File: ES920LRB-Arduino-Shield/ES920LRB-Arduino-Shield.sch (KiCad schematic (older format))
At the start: 18 parts, among them J1 Conn_01x10_Female, J2 Conn_01x12_Female, M1 ES920LR2B, P1 Power, P2 Analog, P3 Digital, P4 Digital, P5 CONN_01X01, P6 CONN_01X01, P7 CONN_01X01, P8 CONN_01X01

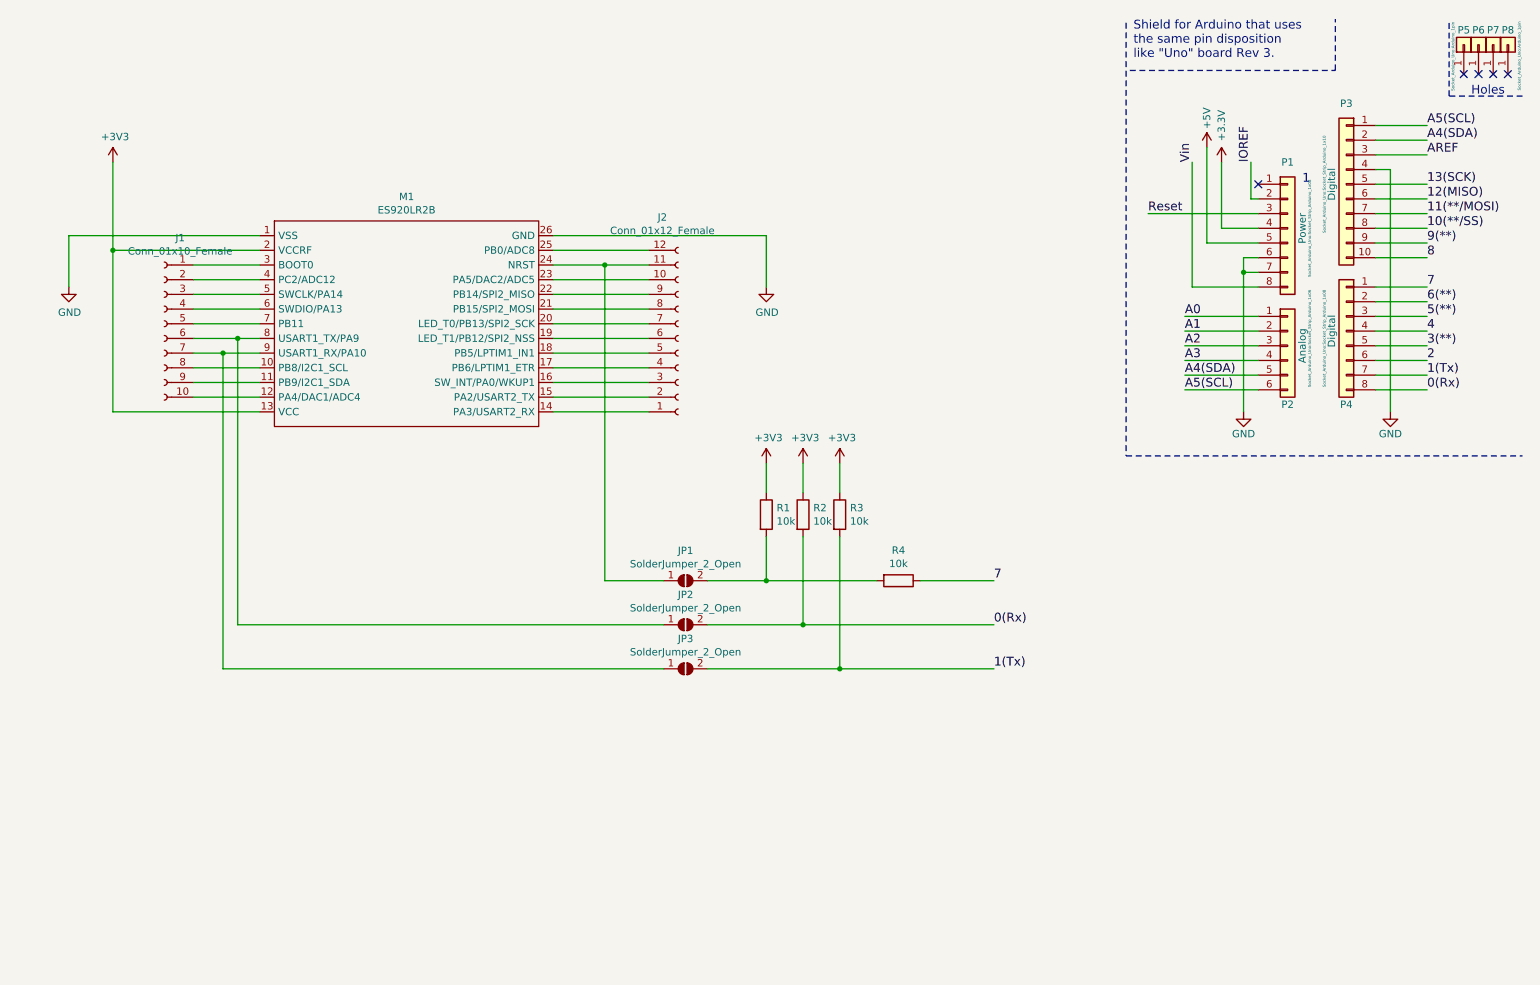
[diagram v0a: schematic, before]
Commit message: add schematica v1.3
add schematica v1.3
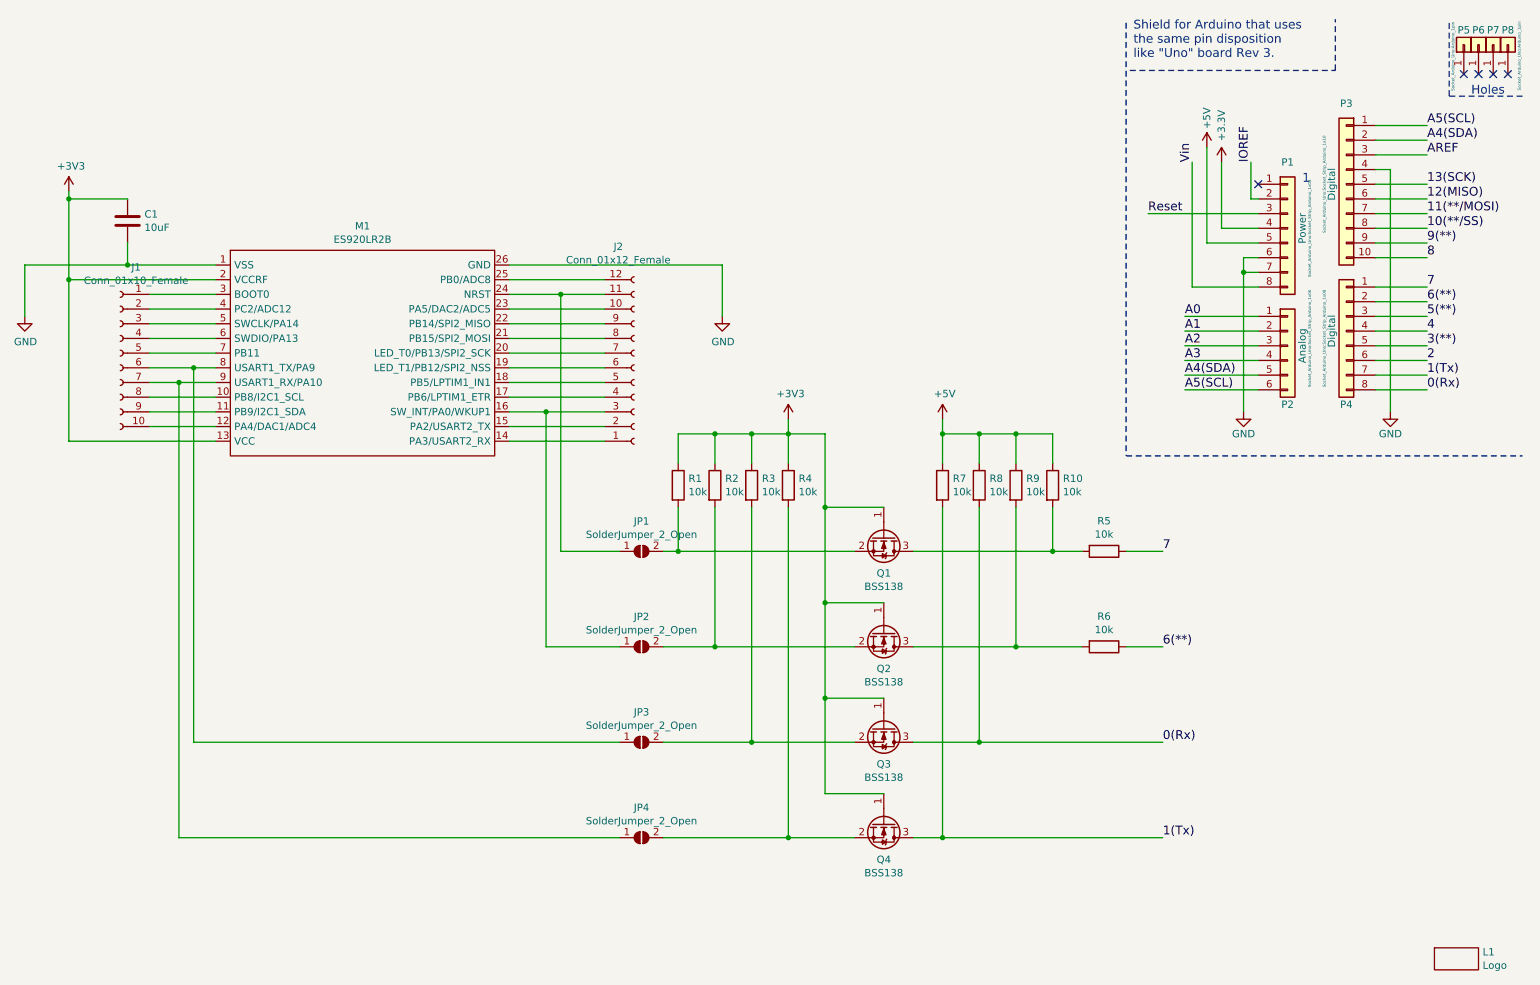
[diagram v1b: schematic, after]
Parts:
- added C1: 10uF, Capacitor_THT:C_Rect_L4.0mm_W2.5mm_P2.50mm, symbol Device:C
- added JP4: SolderJumper_2_Open, Jumper:SolderJumper-2_P1.3mm_Open_Pad1.0x1.5mm, symbol Jumper:SolderJumper_2_Open
- added L1: Logo, teTra:teTra-logo, symbol teTra:Logo
- added Q1, Q2, Q3, Q4: BSS138, Package_TO_SOT_SMD:SOT-23, symbol add_lib2:BSS138
- added R10, R4, R6, R7, R8, R9: 10k, Resistor_THT:R_Axial_DIN0207_L6.3mm_D2.5mm_P2.54mm_Vertical, symbol Device:R
- renumbered R4 to R5
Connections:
- net +3V3: now also C1.1, Q1.1 (G), Q2.1 (G), Q3.1 (G), Q4.1 (G), R4.1
- net +5V: now also R10.1, R7.1, R8.1, R9.1
- net 0(Rx): now also Q3.3 (D), R8.2; no longer JP2.2 (B), R2.2
- net 1(Tx): now also Q4.3 (D), R7.2; no longer JP3.2 (B), R3.2
- net 6(**): now also R6.1
- net GND: now also C1.2
- net at J2.3 (Pin_3), M1.16 (SW_INT/PA0/WKUP1): now also JP2.1 (A)
- net at J1.6 (Pin_6), M1.8 (USART1_TX/PA9): now also JP3.1 (A); no longer JP2.1 (A)
- net at J1.7 (Pin_7), M1.9 (USART1_RX/PA10): now also JP4.1 (A); no longer JP3.1 (A)
- net at JP1.2 (B), R1.2: now also Q1.2 (S); no longer R5.2
- new net: JP2.2 (B), Q2.2 (S), R2.2
- new net: JP3.2 (B), Q3.2 (S), R3.2
- new net: Q1.3 (D), R10.2, R5.2
- new net: JP4.2 (B), Q4.2 (S), R4.2
- new net: Q2.3 (D), R6.2, R9.2
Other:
- moved on the sheet: J1, J2, JP1, JP2, JP3, M1, R1, R2, R3, R5
